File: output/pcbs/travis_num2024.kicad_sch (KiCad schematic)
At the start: 34 parts, among them SW1 SW_Push, SW10 SW_Push, SW11 SW_Push, SW12 SW_Push, SW13 SW_Push, SW14 SW_Push, SW15 SW_Push, SW16 SW_Push, SW17 SW_Push, SW2 SW_Push, SW3 SW_Push, SW4 SW_Push, SW5 SW_Push, SW6 SW_Push, SW7 SW_Push, SW8 SW_Push, SW9 SW_Push

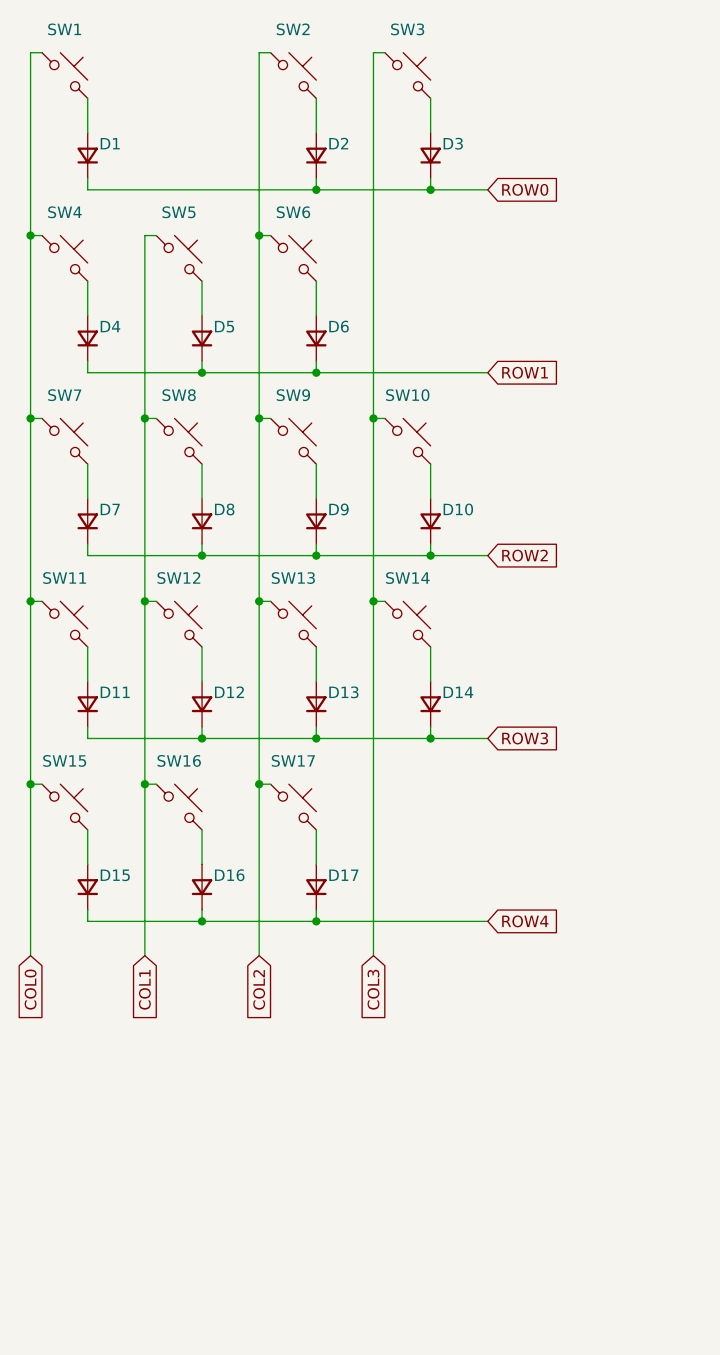
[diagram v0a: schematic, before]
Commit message: numpad cap and firmware
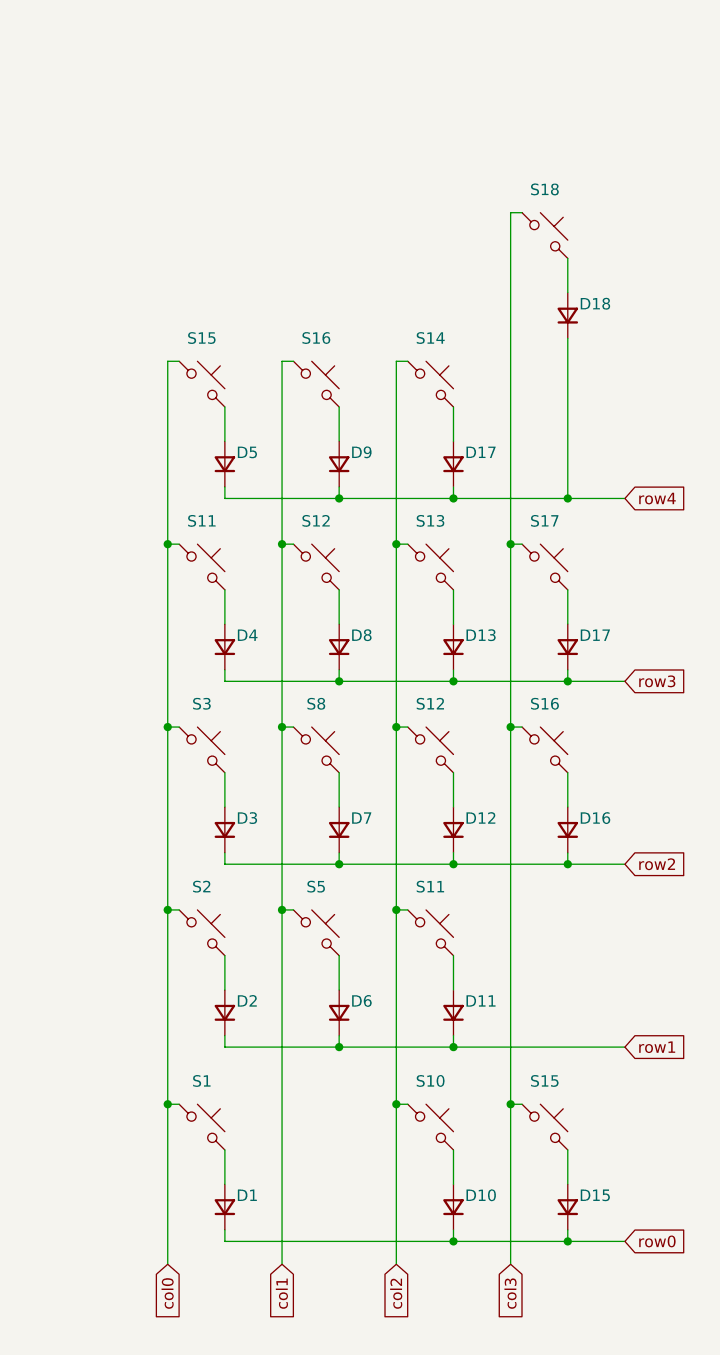
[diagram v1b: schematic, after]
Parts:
- added D18: D, symbol Device:D_Small
- added S18: SW_Push, symbol Switch:SW_Push_45deg
- renumbered D2 to D10, D6 to D11, D9 to D12, D3 to D15, D10 to D16, D14 to D17, D4 to D2, D7 to D3, D11 to D4, D15 to D5, D5 to D6, D8 to D7, D12 to D8, D16 to D9, SW1 to S1, SW2 to S10, SW11 to S11, SW6 to S11, SW9 to S12, SW12 to S12, SW13 to S13, SW17 to S14, SW3 to S15, SW15 to S15, SW10 to S16, SW16 to S16, SW14 to S17, SW4 to S2, SW7 to S3, SW5 to S5, SW8 to S8
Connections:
- net COL0 renamed col0
- net COL1 renamed col1
- net COL2 renamed col2
- net COL3 renamed col3
- net col3: now also S18.1
- net ROW0 renamed row0
- net ROW1 renamed row1
- net ROW2 renamed row2
- net ROW3 renamed row3
- net ROW4 renamed row4
- net row4: now also D18.1 (K)
- new net: D18.2 (A), S18.2
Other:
- moved on the sheet: D1, D10, D11, D12, D13, D15, D16, D17, D2, D3, D4, D5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
